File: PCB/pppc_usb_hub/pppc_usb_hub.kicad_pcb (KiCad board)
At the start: 2 copper layers, 69.6 x 48 mm, 83 parts, among them J1 USB_C_Signal, J2 USB_C_Signal, J3 USB_A_1, J4 USB_A_2, J5 USB_A_3, J6 Con_Relay, J7 Conn_UART, J8 Conn_Debug, K1 Relay, Q1 DMG2305UX, Q2 DMMT5401, Q3 AO3400A, SW1 USB1, SW2 USB2, SW3 USB3, SW4 BOOT0, SW5 RESET, U1 MT9700, U2 MT9700, U3 MT9700, U4 SL2.1s, U5 AMS1117-3.3, U6 STM32F042F6Px

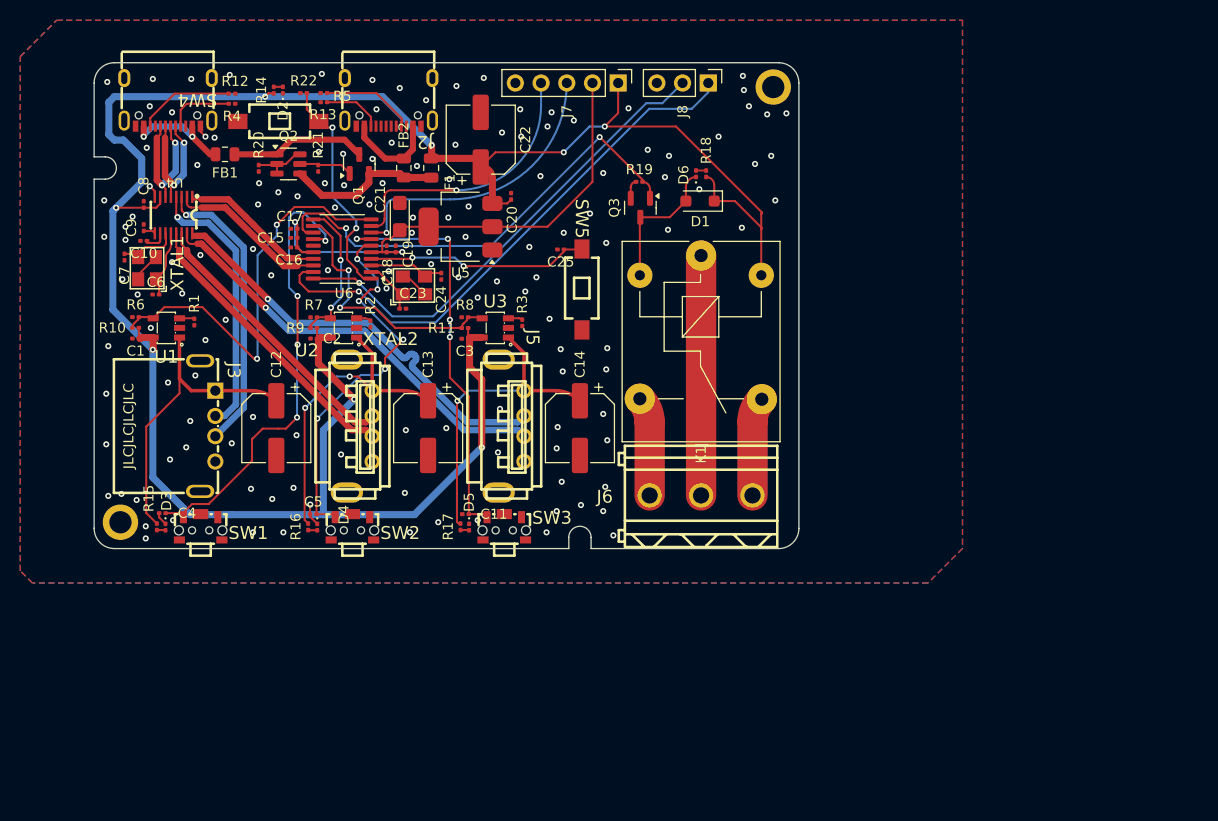
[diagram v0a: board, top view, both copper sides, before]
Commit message: Rev 2
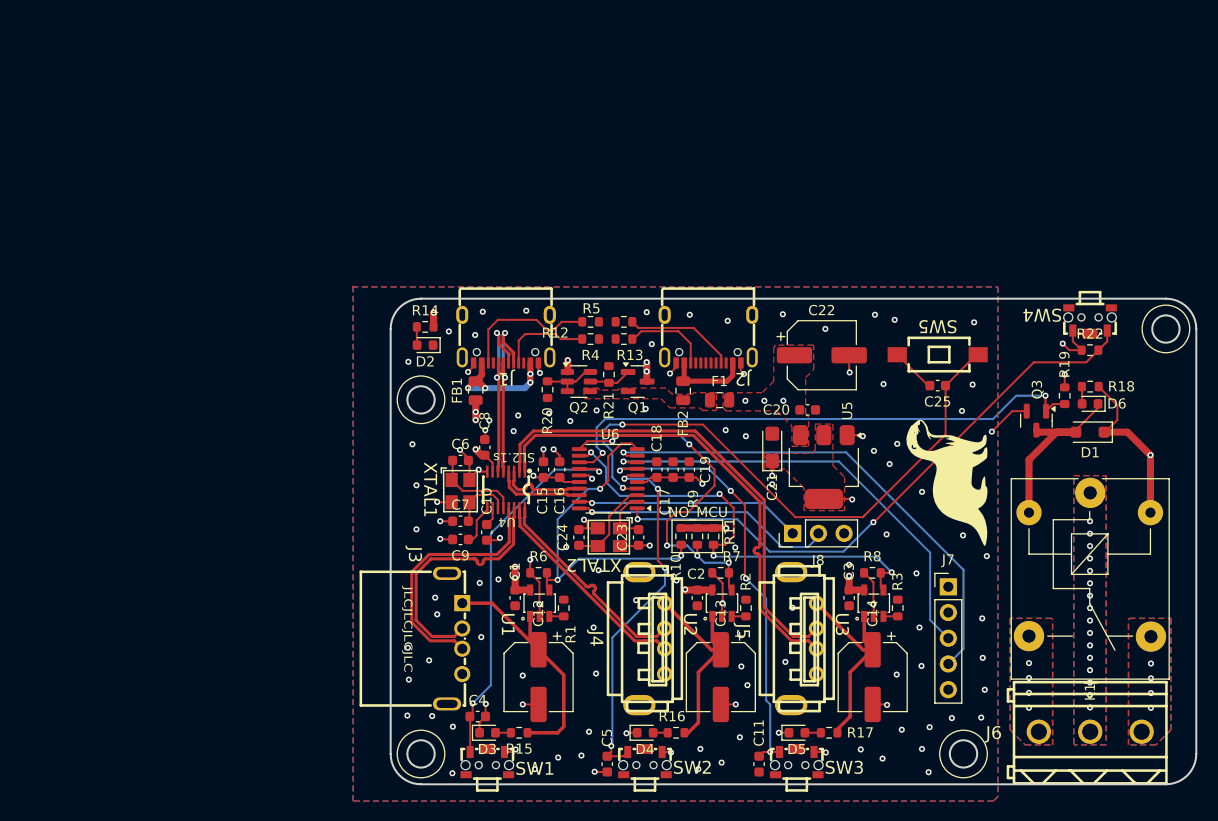
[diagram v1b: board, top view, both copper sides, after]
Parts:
- removed REF** (x2): MountingHole_2.2mm_M2_ISO7380_Pad, MountingHole:MountingHole_2.2mm_M2_ISO7380_Pad
- added G***: LOGO, LOGO, F.Cu at (163.7, 98.7)
- C1, C10, C11, C15, C16, C17, C18, C19, C2, C20, C23, C24, C25, C3, C4, C5, C6, C7, C8, C9: footprint Capacitor_SMD:C_0201_0603Metric -> Capacitor_SMD:C_0603_1608Metric
- D2, D3, D4, D5, D6: footprint LED_SMD:LED_0201_0603Metric -> LED_SMD:LED_0603_1608Metric
- R1, R10, R11, R12, R13, R14, R15, R16, R17, R18, R19, R2, R20, R21, R22, R3, R4, R5, R6, R7, R8, R9: footprint Resistor_SMD:R_0201_0603Metric -> Resistor_SMD:R_0603_1608Metric
- SW4: footprint PCBLIB_SW-SMD_L6.0-W3.3-LS8.0_2024-05-19:SW-SMD_L6.0-W3.3-LS8.0 -> PCBLIB_SW-SMD_GT-TC020B-H035-L05_2024-05-21:SW-SMD_GT-TC020B-H035-L05
- moved SW4 82.6 mm to (177.8, 83.2)
- moved R22 81.7 mm to (177.8, 86.1)
- moved J7 59.5 mm to (163.8, 109.5), turned to 0 degrees
- moved R10 57.7 mm to (137.4, 104.5), turned to -90 degrees
- moved R8 47.5 mm to (156.3, 108.1)
- moved R7 47.5 mm to (141.3, 108.1)
- moved R6 47.2 mm to (123.3, 108.1)
- moved R19 47.0 mm to (175.3, 90.6), turned to 90 degrees
- moved R3 46.6 mm to (158.8, 111.6), turned to 90 degrees
- moved R2 46.5 mm to (143.8, 111.6), turned to 90 degrees
- moved U2 46.2 mm to (141.4, 111.1), turned to -90 degrees
- moved U3 46.2 mm to (156.4, 111.1), turned to -90 degrees
- moved R1 46.2 mm to (125.8, 111.6), turned to 90 degrees
- moved U1 45.8 mm to (123.4, 111.1), turned to -90 degrees
- moved C3 45.8 mm to (154.0, 110.6), turned to -90 degrees
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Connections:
- U4 pad 1: /MCU_DN -> /DN3
- U4 pad 13: /DN2 -> /DN1
- U4 pad 14: /DP2 -> /DP1
- U4 pad 15: /DN3 -> /DN2
- U4 pad 16: /DP3 -> /DP2
- U4 pad 2: /MCU_DP -> /DP3
- U4 pad 3: /DN1 -> /MCU_DN
- U4 pad 4: /DP1 -> /MCU_DP
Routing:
- net GND: track 13.8 -> 90.8 mm, vias 141 -> 118
- net /NRST: track 22.1 -> 58.5 mm
- net /BOOT0: track 22.6 -> 58.5 mm
- net /VBUS: track 225.6 -> 191.0 mm, vias 8 -> 13
- net /SWDIO: track 54.5 -> 22.4 mm
- net /COM: track 23.7 -> 0.00 mm, vias 0 -> 16
- net /UART_RX: track 26.4 -> 49.8 mm
- net /SWCLK: track 47.6 -> 26.0 mm
- net /EN2: track 14.6 -> 36.2 mm, vias 2 -> 5
- net /EN3: track 26.5 -> 46.1 mm, vias 2 -> 4
- net /UART_TX: track 28.4 -> 44.6 mm
- net VEXT: track 15.5 -> 0.00 mm
- net VUSB: track 13.5 -> 27.0 mm, vias 0 -> 5
- net /VBUS2: track 31.7 -> 21.0 mm, vias 2 -> 0
- net /VBUS3: track 31.1 -> 20.7 mm, vias 1 -> 0
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- added copper zone on F.Cu, net +3.3V
- added copper zone on B.Cu, net /COM
- added copper zone on F.Cu, net /COM
- added copper zone on In1.Cu, net /COM
- added copper zone on In2.Cu, net /COM
- added copper zone on B.Cu, net /NC
- added copper zone on F.Cu, net /NC
- added copper zone on In1.Cu, net /NC
- added copper zone on In2.Cu, net /NC
- added copper zone on B.Cu, net /NO
- added copper zone on F.Cu, net /NO
- added copper zone on In1.Cu, net /NO
- added copper zone on In2.Cu, net /NO
- added copper zone on F.Cu, net /VBUS
- added copper zone on In2.Cu, net /VBUS
- added copper zone on In1.Cu, net GND
- added copper zone on In2.Cu, net GND
- added copper zone on F.Cu, net VEXT
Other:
- board size 69.6 x 48 mm -> 79.6 x 48 mm
- copper layers 2 -> 4
- board text added: "NO_MCU"
